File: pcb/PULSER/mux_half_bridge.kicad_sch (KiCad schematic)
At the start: 12 parts, among them Q16 N-ch, Vds>=200V, fast switch,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, Q17 N-ch, Vds>=200V, fast switch,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, U10 IR2104S

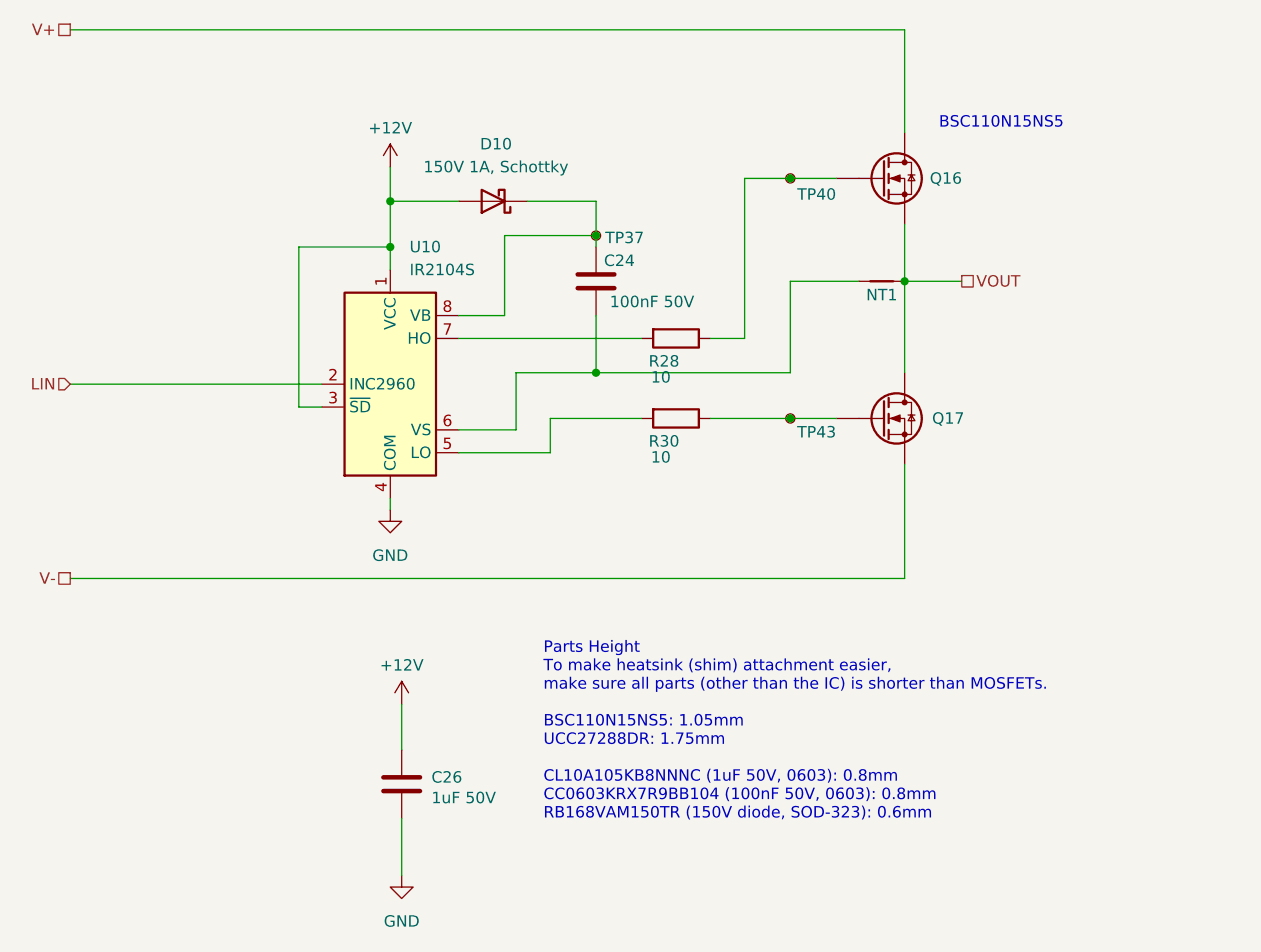
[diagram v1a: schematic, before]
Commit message: EMI reduction & heatsink simplification
EMI: MOSFET snubber, 36V pi-filter
heatsink: Parallel mux bridge
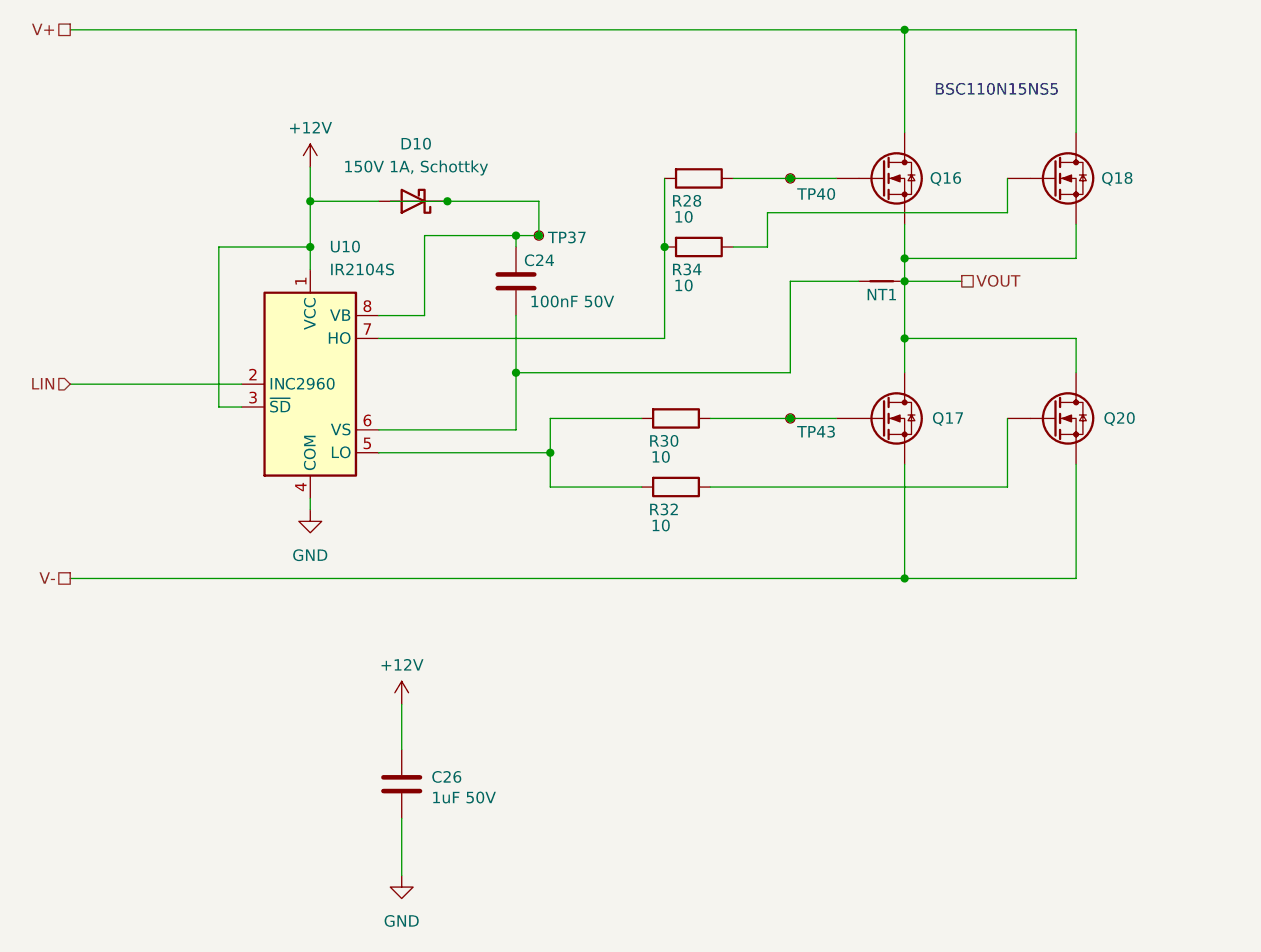
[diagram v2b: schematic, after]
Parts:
- added Q18, Q20: N-ch, Vds>=200V, fast switch, low Rds, SparkAll:Infineon-TG-TDSON-8-NMOS, symbol Device:Q_NMOS
- added R32, R34: 10, Resistor_SMD:R_0603_1608Metric, symbol Device:R
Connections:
- net V+: now also Q18.D
- net V-: now also Q20.S
- net VOUT: now also Q18.S, Q20.D
- net at R30.2, U10.5 (LO): now also R32.2
- net at R28.2, U10.7 (HO): now also R34.2
- new net: Q18.G, R34.1
- new net: Q20.G, R32.1
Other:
- note removed: "Parts Height To make heatsink (shim) attachment easier, make sure all parts (other than the IC) is shorter than MOSFETs. BSC110N15NS5: 1.05mm UCC27288DR: 1.75mm CL10A105KB8NNNC (1uF 50V, 0603): 0.8mm CC0603KRX7R9BB104 (100nF 50V, 0603): 0.8mm RB168VAM150TR (150V diode, SOD-323): 0.6mm"
- moved on the sheet: C24, D10, R28, TP37, U10
